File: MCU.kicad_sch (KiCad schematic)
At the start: 16 parts, among them U10 MCP23017_ML, U11 ESP32-C6-WROOM-1, U12 KMR241GLFS, U13 KMR241GLFS, U5 CD74HC4067M, Y1 32.768kHz 9pF

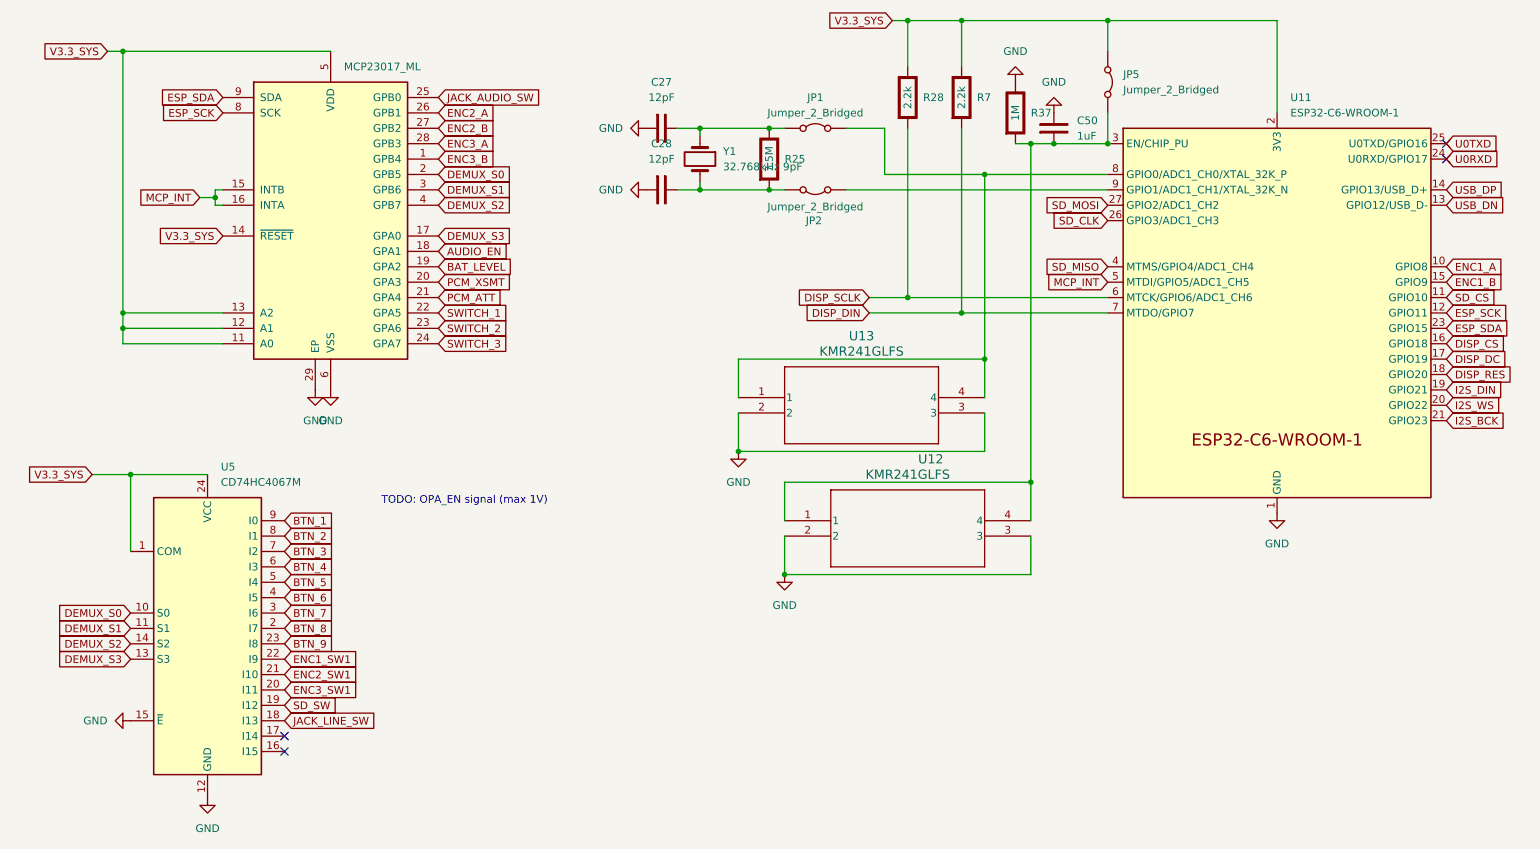
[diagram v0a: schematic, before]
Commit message: routing
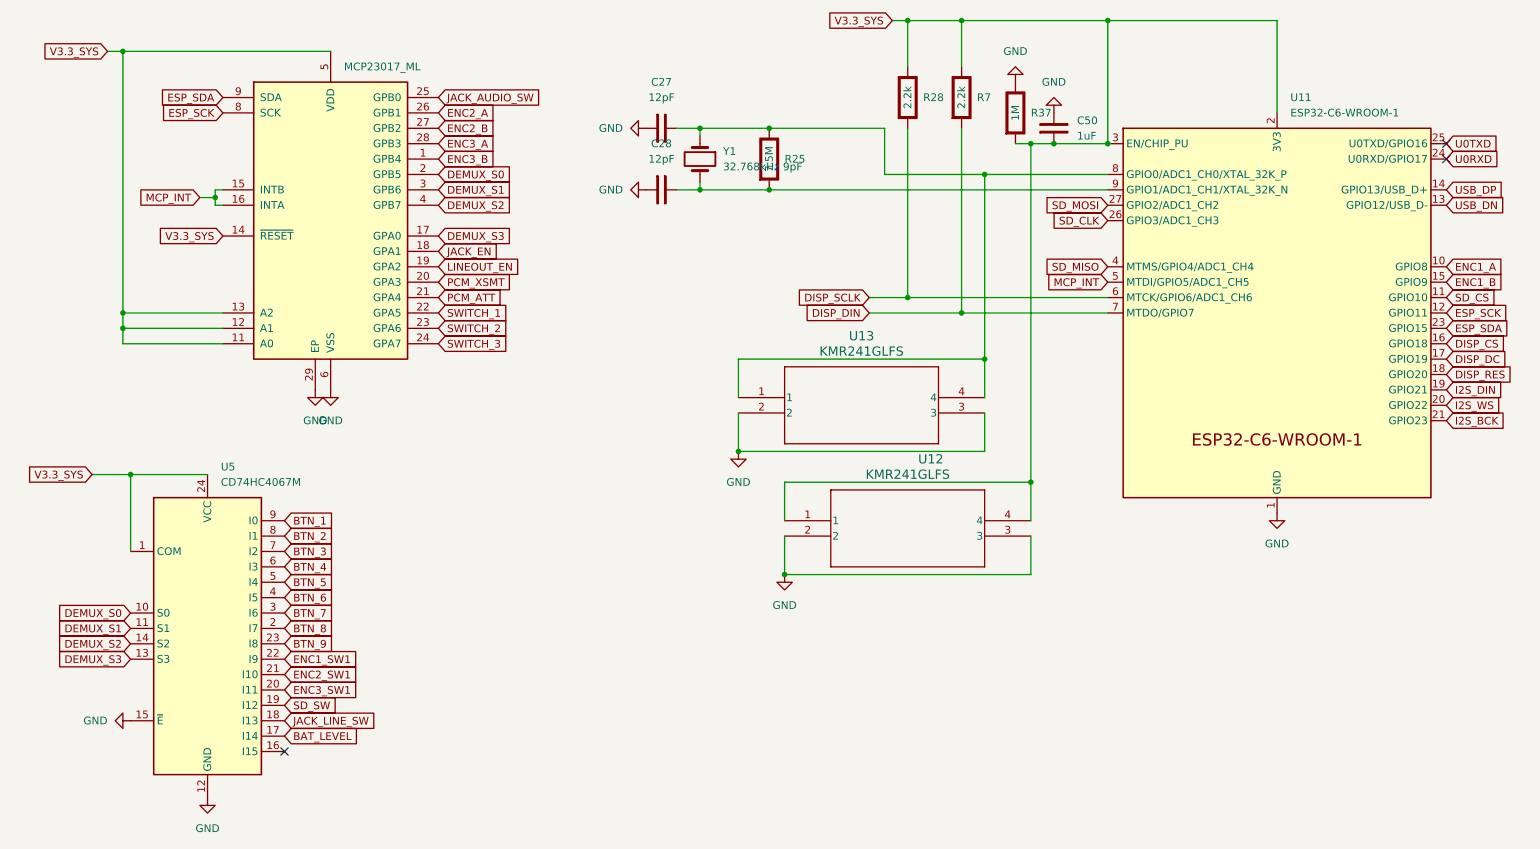
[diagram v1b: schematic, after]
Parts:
- removed JP1, JP2, JP5: Jumper_2_Bridged, PCM_Jumper_AKL:Jumper_P2.54mm_D0.7mm, symbol Jumper:Jumper_2_Bridged
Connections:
- net BAT_LEVEL: now also U5.17 (I14); no longer U10.19 (GPA2)
- net V3.3_SYS: now also C50.1, R37.2 (-), U11.3 (EN/CHIP_PU), U12.1, U12.4
- net at C27.2, R25.1 (+), Y1.1: now also U11.8 (GPIO0/ADC1_CH0/XTAL_32K_P), U13.1, U13.4
- net at C28.2, R25.2 (-), Y1.2: now also U11.9 (GPIO1/ADC1_CH1/XTAL_32K_N)
- net AUDIO_EN renamed JACK_EN
- new net LINEOUT_EN: U10.19 (GPA2)
- no-connect marks 4 -> 3
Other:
- note removed: "TODO: OPA_EN signal (max 1V)"
